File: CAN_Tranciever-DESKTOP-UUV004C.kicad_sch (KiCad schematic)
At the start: 5 parts, among them J4 Conn_01x02_Socket, U4 MCP2542WFDxMF (CAN)

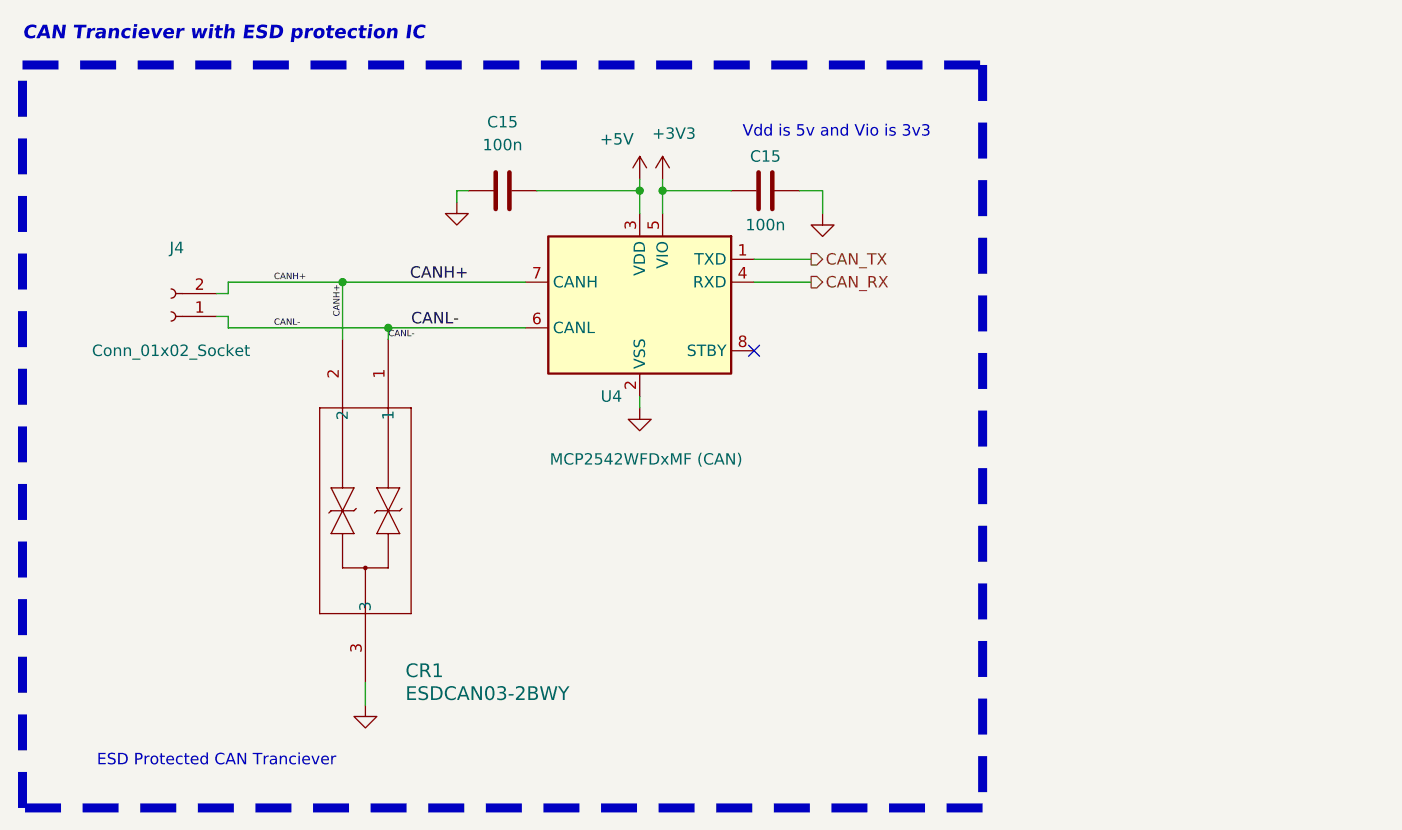
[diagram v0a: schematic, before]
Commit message: Done power
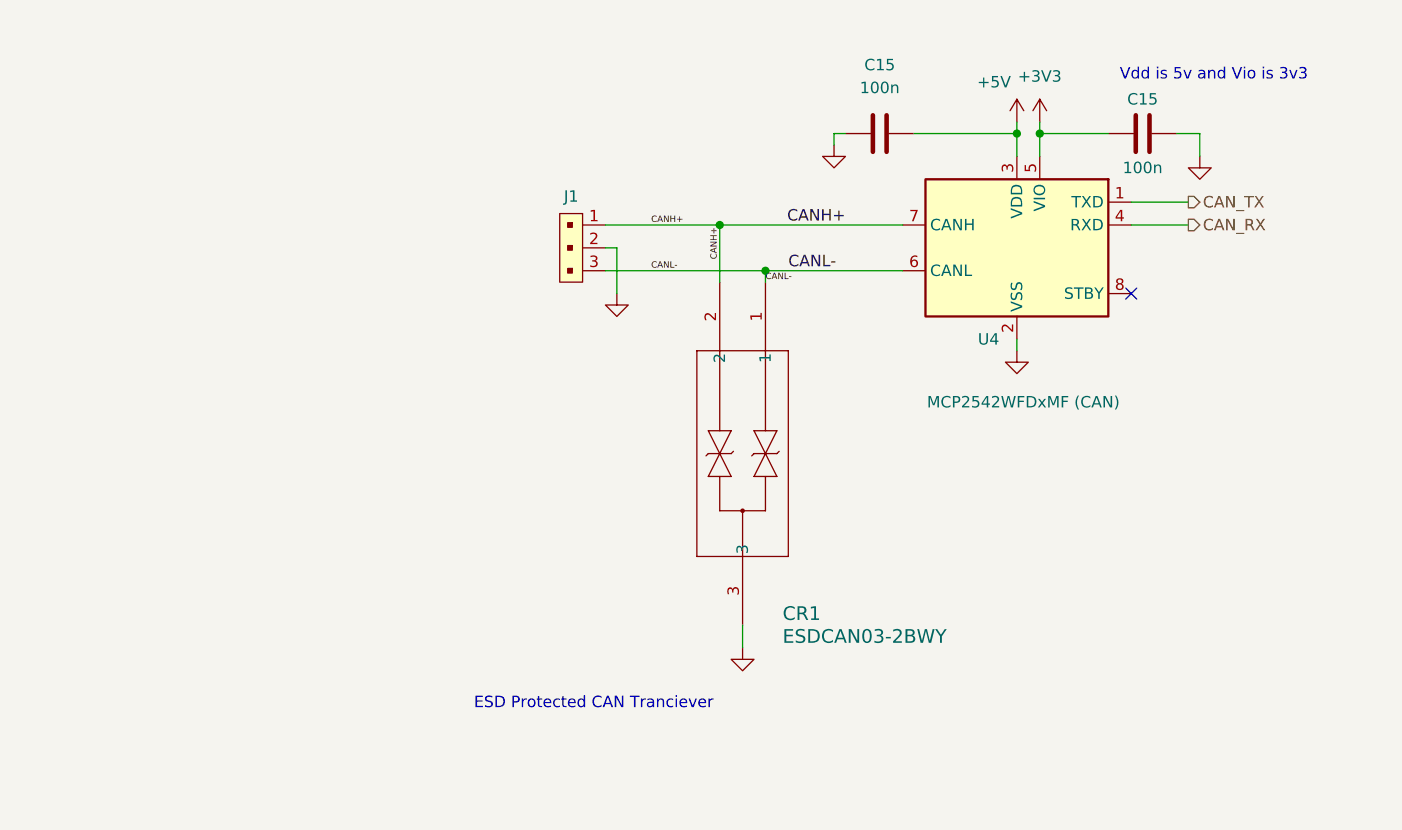
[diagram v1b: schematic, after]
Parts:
- removed J4: Conn_01x02_Socket, Connector_PinHeader_2.54mm:PinHeader_1x02_P2.54mm_Vertical, symbol Connector:Conn_01x02_Socket
- added J1: 0022232031, digikey-footprints:PinHeader_1x3_P2.54mm_Drill1.02mm, symbol dk_Rectangular-Connectors-Headers-Male-Pins:0022232031
- CR1: JLC # C1973833 -> (none)
- U4: JLC # C191252 -> (none)
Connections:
- net CANH+: now also J1.1
- net CANL-: now also J1.3
- net GND: now also J1.2
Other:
- note removed: "CAN Tranciever with ESD protection IC"
- moved on the sheet: C15, CR1, U4
